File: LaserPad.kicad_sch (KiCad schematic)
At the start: 7 parts, among them U1 STM32F072C8Tx, U3 PRTR5V0U2X, U4 USBLC6-2SC6

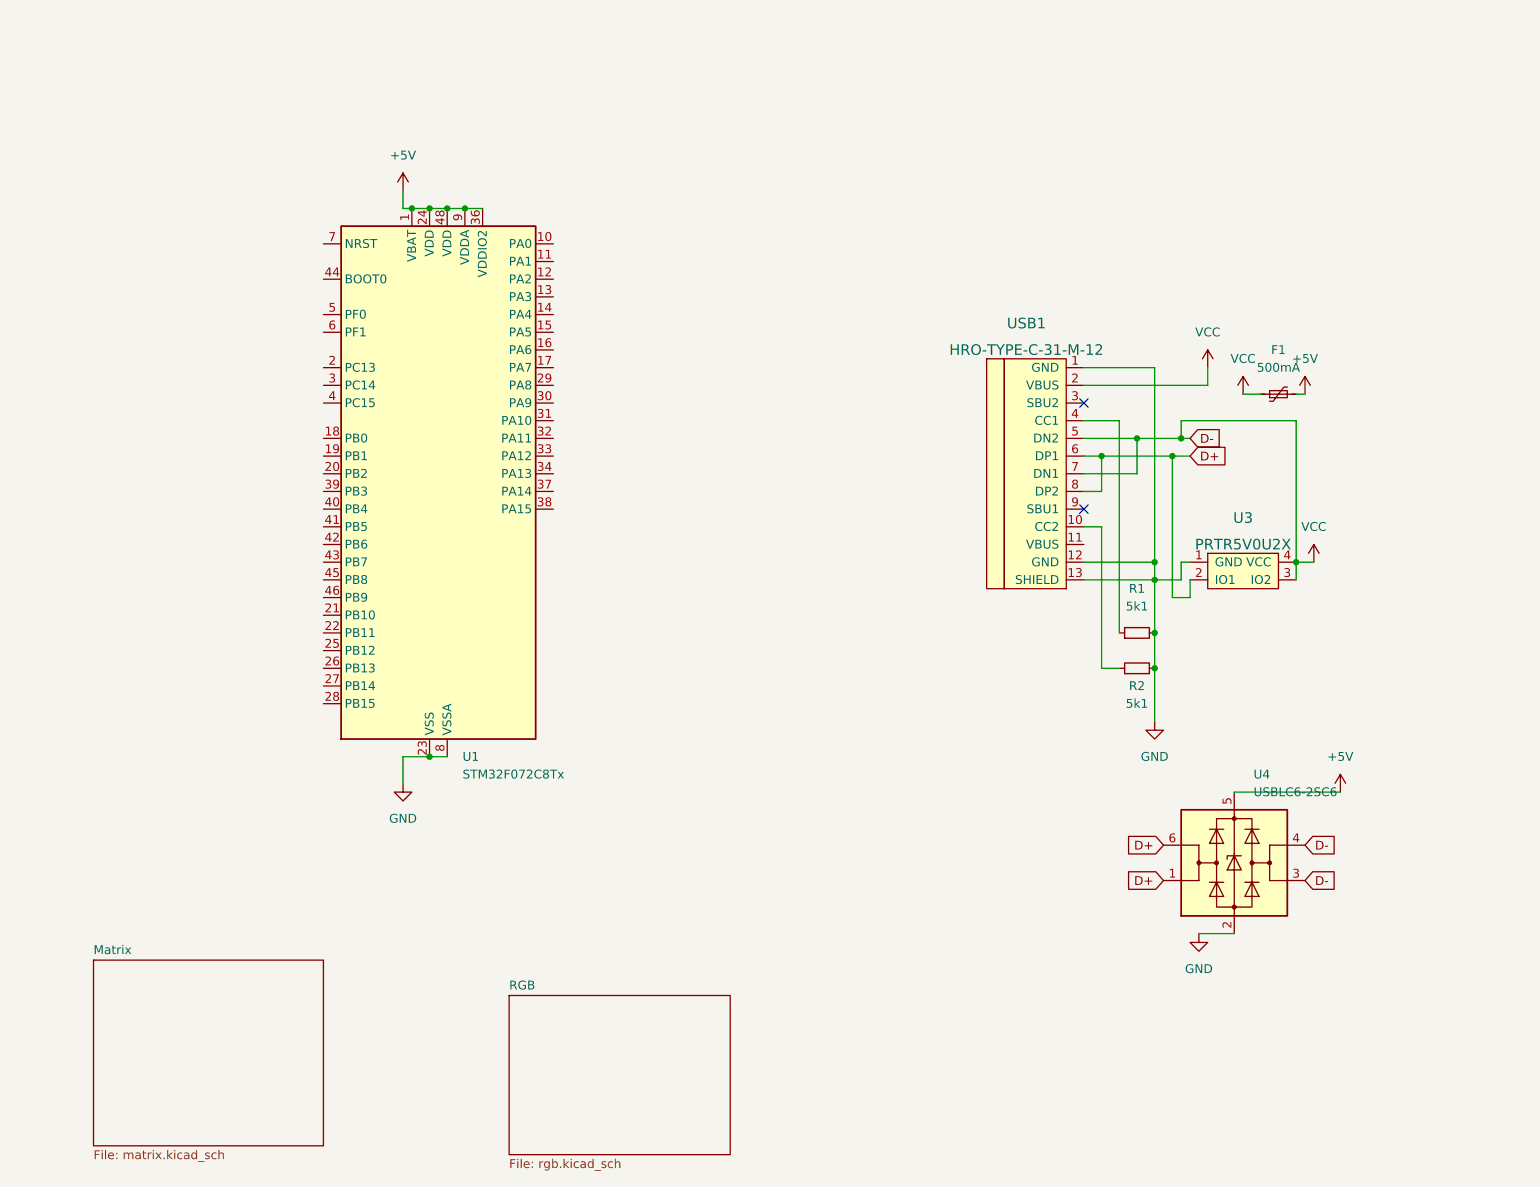
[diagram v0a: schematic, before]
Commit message: did a little organization :/
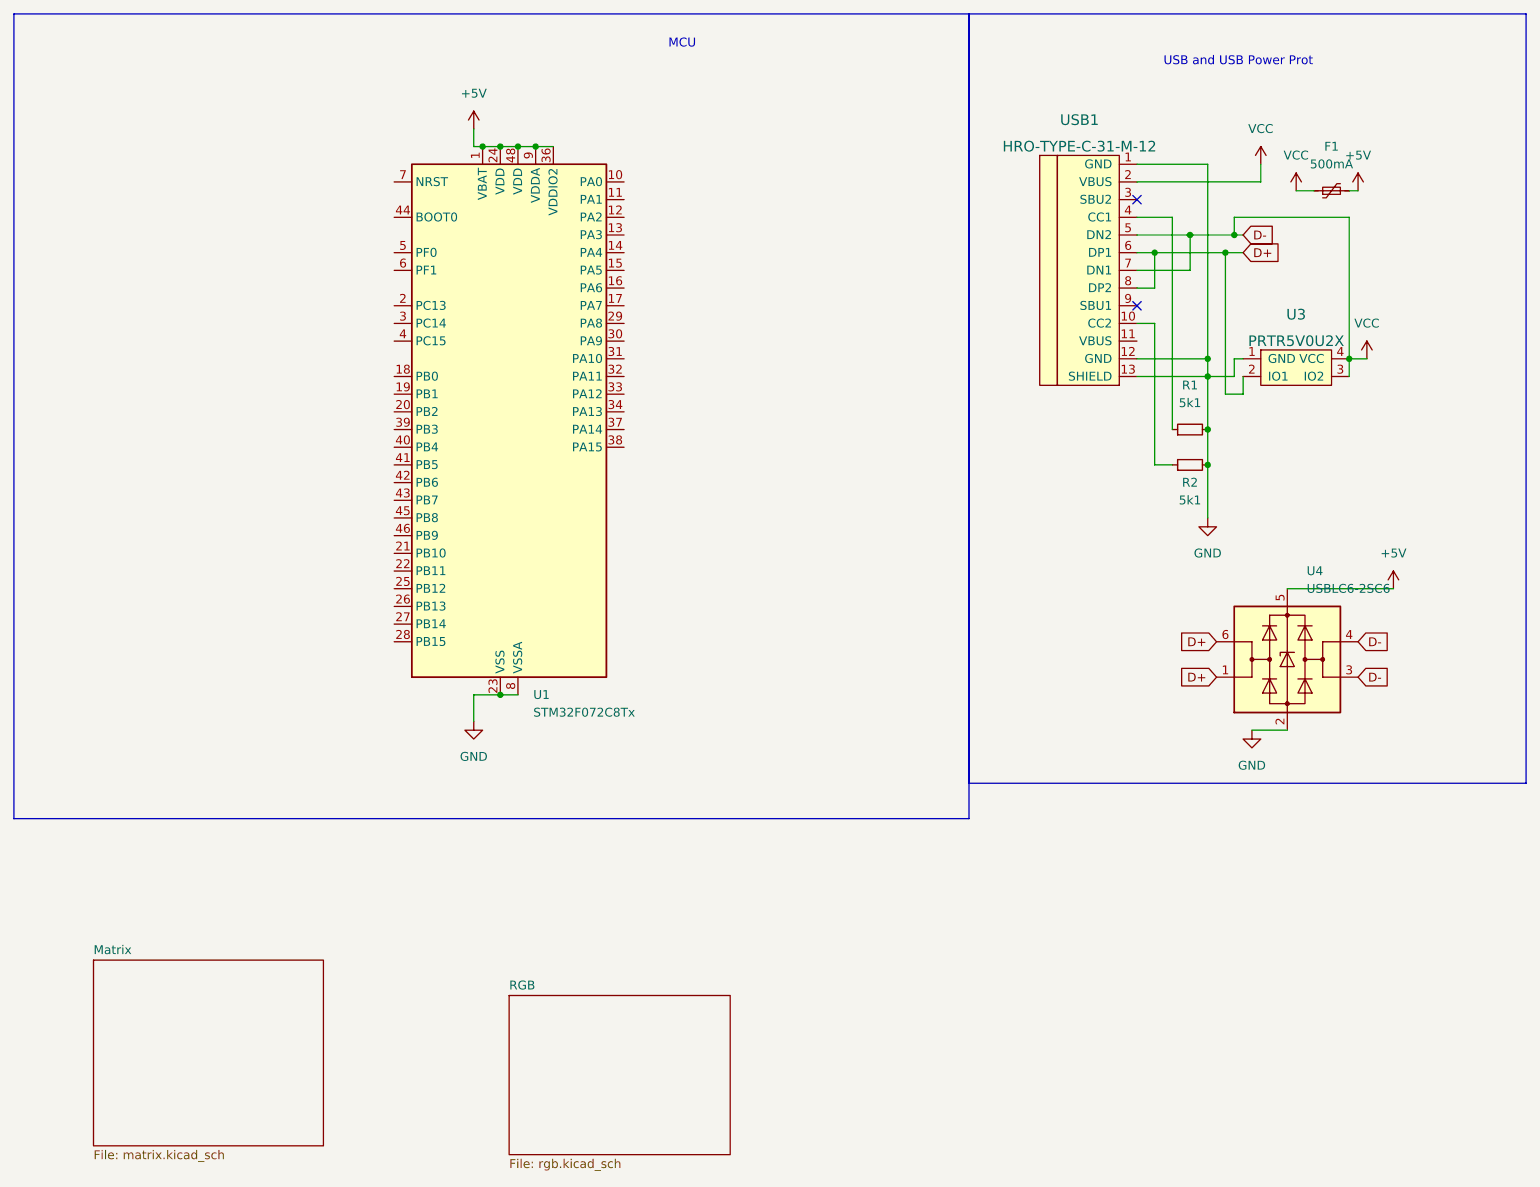
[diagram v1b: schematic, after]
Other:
- note added: "MCU"
- note added: "USB and USB Power Prot"
- moved on the sheet: F1, R1, R2, U1, U3, U4, USB1
